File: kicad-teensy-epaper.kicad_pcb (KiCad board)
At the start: 2 copper layers, 69 x 42.4 mm, 18 parts, among them J1 TEENSY3.2-72MHz, J2 HEADER-FEMALE-34POS-FFC-SMT-1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, Q1 Q_NMOS_GDS

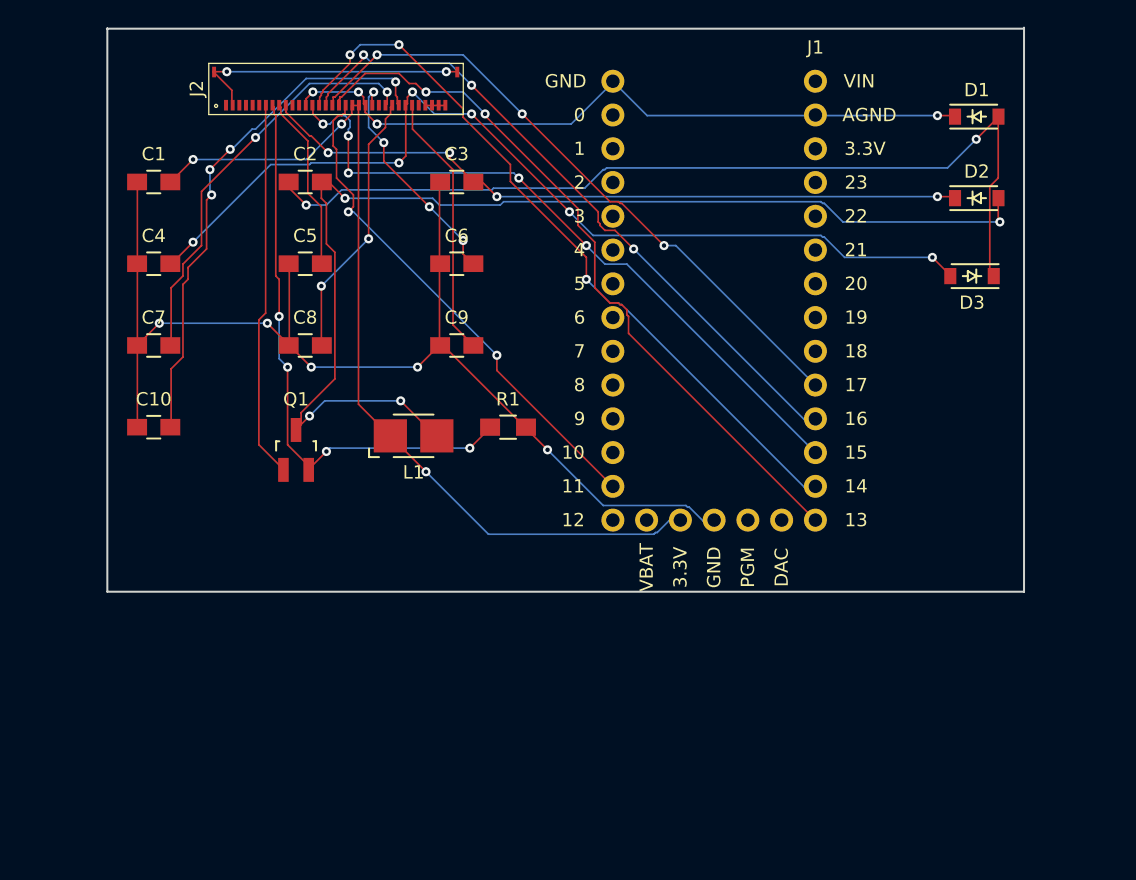
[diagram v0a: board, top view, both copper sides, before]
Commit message: order new version
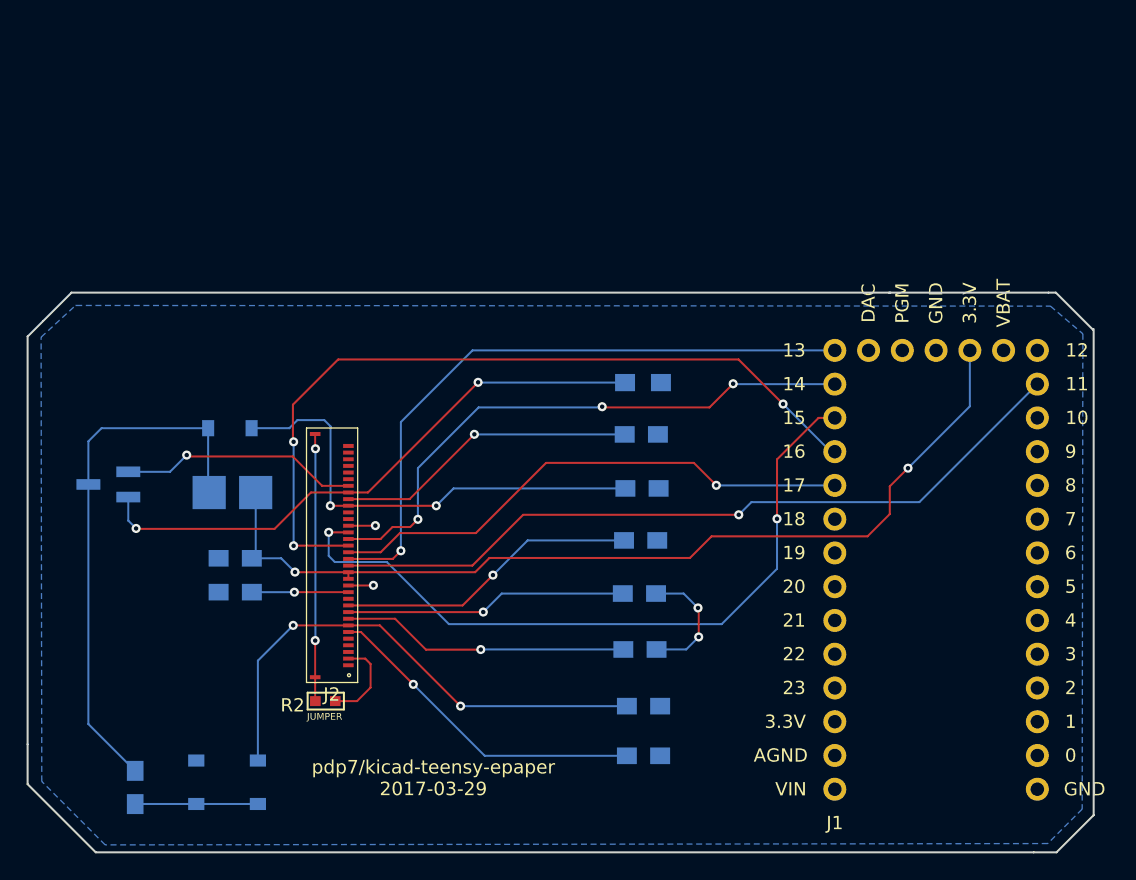
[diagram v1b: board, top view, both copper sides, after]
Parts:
- added R2: RES-0.0-JUMPER-1/8W-0603, RLC-0603-SMD, F.Cu at (111.8, 74.0)
- C1, C10, C2, C3, C4, C5, C6, C7, C8, C9, D1, D2, D3, L1, Q1, R1: moved to B.Cu
- moved D1 77.2 mm to (102.1, 80.1), turned to 270 degrees
- moved D3 65.9 mm to (106.7, 80.1), turned to 90 degrees
- moved D2 58.8 mm to (104.6, 53.5), turned to 180 degrees
- moved C4 49.7 mm to (135.7, 74.4), turned to 180 degrees
- moved C2 47.3 mm to (97.5, 80.5), turned to 90 degrees
- moved C10 40.2 mm to (135.5, 70.1), turned to 180 degrees
- moved C7 39.5 mm to (135.5, 61.9), turned to 180 degrees
- moved J2 35.1 mm to (112.4, 63.1), turned to 90 degrees
- moved J1 34.9 mm to (155.2, 70.5), turned to 180 degrees
- moved C9 33.9 mm to (135.7, 78.1), turned to 180 degrees
- moved C8 31.3 mm to (135.4, 65.9), turned to 180 degrees
- moved C6 29.8 mm to (105.0, 65.8)
- moved C1 29.0 mm to (105.0, 63.3)
- moved C5 28.4 mm to (135.6, 54.0), turned to 180 degrees
- moved C3 26.9 mm to (135.6, 58.0), turned to 180 degrees
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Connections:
- net BS1 renamed GND
- net NC1 renamed Net-(J2-Pad1)
- net NC3 renamed Net-(J2-Pad3)
- net NC4 renamed Net-(J2-Pad4)
- net NC5 renamed Net-(J2-Pad5)
- net NC7 renamed Net-(J2-Pad30)
- J2 pad 10: VGH -> VSH
- J2 pad 11: TSCL -> VPP
- J2 pad 12: TSDA -> VDD
- J2 pad 14: BUSY -> VDDIO
- J2 pad 15: ^RES -> VDDIO
- J2 pad 16: ^D/C -> DOUT
- J2 pad 17: ^CS -> SCK
- J2 pad 18: SCK -> ^CS
- J2 pad 19: DOUT -> ^D/C
- J2 pad 2: NC2 -> Net-(J2-Pad2)
- J2 pad 20: VDDIO -> ^RES
- J2 pad 21: VDDIO -> BUSY
- J2 pad 23: VDD -> TSDA
- J2 pad 24: VPP -> TSCL
- J2 pad 25: VSH -> VGH
- J2 pad 26: VGH2 -> VGL
- J2 pad 27: VSL -> RESE
- J2 pad 28: PRVGL -> GDR
- J2 pad 29: VCOM -> Net-(J2-Pad29)
- J2 pad 31: NC8 -> Net-(J2-Pad31)
- J2 pad 32: NC8 -> Net-(J2-Pad32)
- J2 pad 33: NC8 -> Net-(J2-Pad33)
- J2 pad 34: NC8 -> Net-(J2-Pad34)
- J2 pad 6: NC6 -> VCOM
- J2 pad 7: GDR -> PRVGL
- J2 pad 8: RESE -> VSL
- J2 pad 9: VGL -> VGH2
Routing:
- net GND: track 143.5 -> 13.3 mm, vias 9 -> 4
- net Net-(C2-Pad1): track 69.6 -> 9.24 mm, vias 2 -> 0
- net Net-(C2-Pad2): track 87.5 -> 40.5 mm, vias 4 -> 0
- net PRVGL: track 72.5 -> 38.9 mm, vias 6 -> 2
- net Net-(J2-Pad2): track 0.00 -> 26.8 mm, vias 0 -> 2
- net NC2: track 21.8 -> 0.00 mm, vias 2 -> 0
- net DOUT: track 38.7 -> 57.5 mm, vias 2 -> 1
- net VGH: track 53.9 -> 35.1 mm, vias 4 -> 2
- net VSL: track 39.6 -> 21.7 mm, vias 4 -> 1
- net ^RES: track 56.1 -> 43.7 mm
- net GDR: track 28.5 -> 18.0 mm, vias 0 -> 1
- net VDD: track 17.5 -> 7.26 mm, vias 4 -> 1
- net VGL: track 13.3 -> 22.8 mm, vias 0 -> 1
- net ^D/C: track 51.0 -> 59.8 mm
- net ^CS: track 48.7 -> 40.1 mm, vias 3 -> 1
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- added copper zone on B.Cu, net GND
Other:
- board size 69 x 42.4 mm -> 80.2 x 42.1 mm
- net class Default: clearance 0.127 -> 0.1524; trace_width 0.127 -> 0.1524
- rule trace_clearance: 0.127 -> 0.1524
- rule trace_min: 0.127 -> 0.1524
- board text added: "JUMPER"
- board text added: "pdp7/kicad-teensy-epaper 2017-03-29"
